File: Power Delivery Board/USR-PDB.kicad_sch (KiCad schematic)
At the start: 35 parts, among them U1 XT90, U10 Anderson PP45 Vert. 2x1, U11 Anderson PP45 Vert. 2x1, U12 Anderson PP45 Vert. 2x1, U13 LM2575-5.0BT, U14 MCP3002-I/P, U2 Anderson PP45 Vert. 2x1, U3 Anderson PP45 Vert. 2x1, U4 Anderson PP45 Vert. 2x1, U5 Anderson PP45 Vert. 2x1, U6 Anderson PP45 Vert. 2x1, U7 LM2676T-12_NOPB

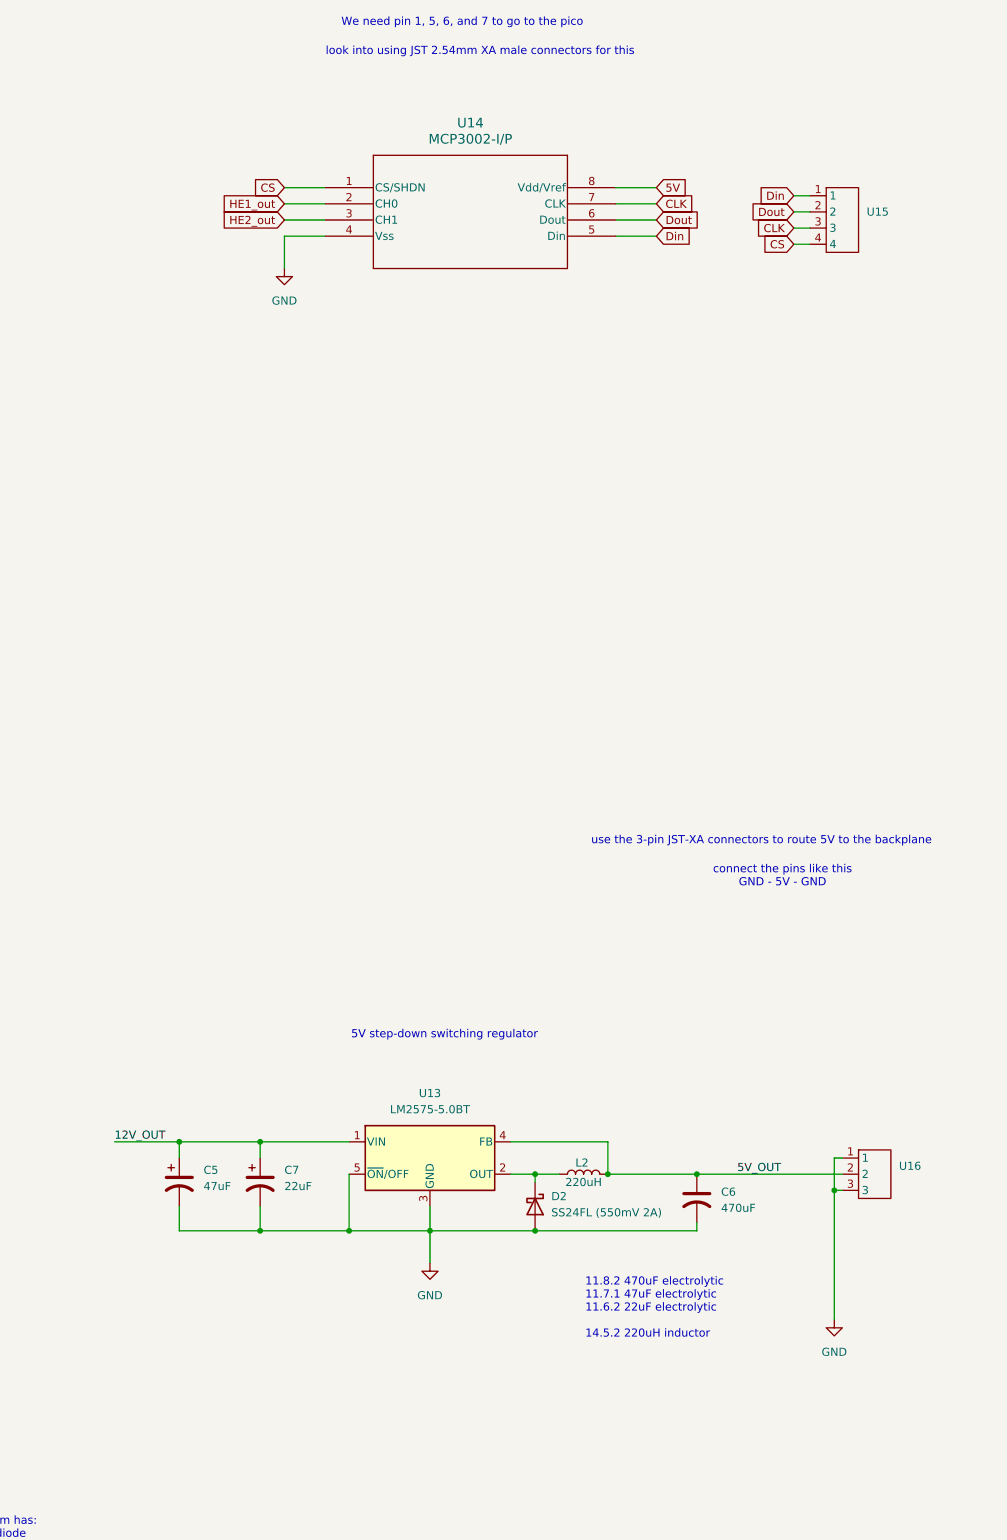
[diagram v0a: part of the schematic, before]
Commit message: updated PDB and analog board
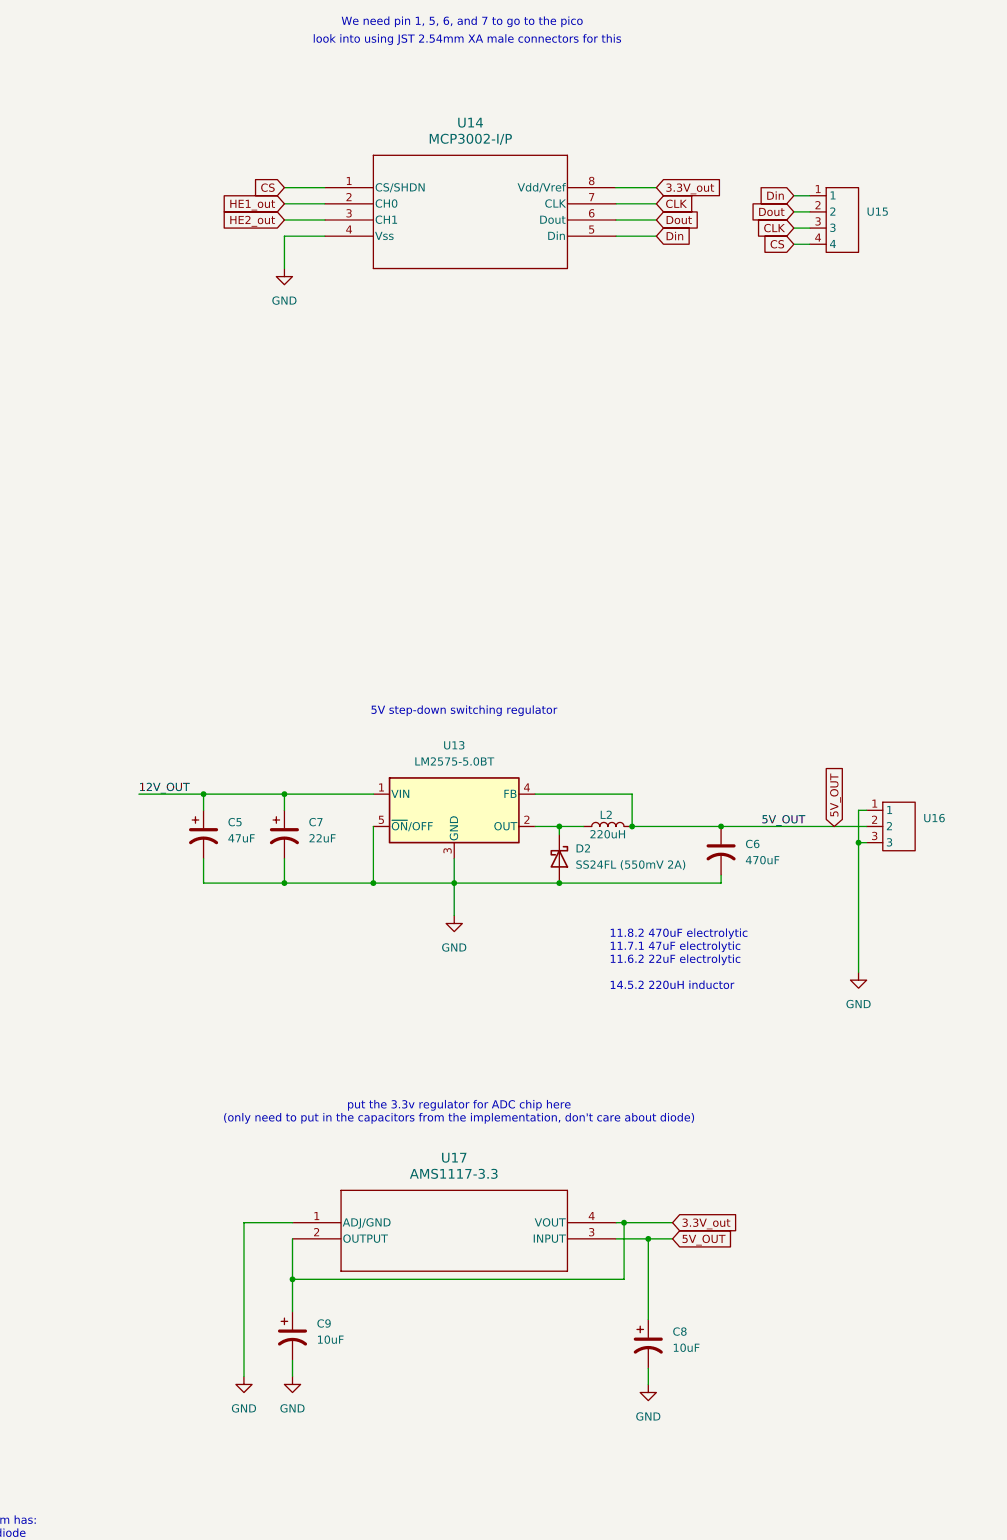
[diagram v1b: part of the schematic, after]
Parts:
- added C8, C9: 10uF, Capacitor_SMD:C_0805_2012Metric_Pad1.18x1.45mm_HandSolder, symbol Device:C_Polarized_US
- added U17: AMS1117-3.3, USR:SOT_AMS1117-2.5_AMS, symbol USR:AMS1117-3.3
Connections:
- net 5V_OUT: now also C8.1, U17.3 (INPUT)
- net GND: now also C8.2, C9.2, U17.1 (ADJ/GND)
- net 5V renamed 3.3V_out
- net 3.3V_out: now also C9.1, U17.2 (OUTPUT), U17.4 (VOUT)
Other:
- note added: "put the 3.3v regulator for ADC chip here (only need to put in the capacitors from the implementation, don't care about diode)"
- note removed: "connect the pins like this GND - 5V - GND"
- note removed: "use the 3-pin JST-XA connectors to route 5V to the backplane"
- moved on the sheet: C5, C6, C7, D2, L2, U13, U16
